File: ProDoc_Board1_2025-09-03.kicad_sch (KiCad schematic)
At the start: 47 parts, among them CN10 BATT, CN11 CHGIN, CN2 B04B-XNISK-A-1(LF)(SN), CN3 B04B-XNISK-A-1(LF)(SN), CN4 B04B-XNISK-A-1(LF)(SN), CN7 XH2.54-5PIN, CN8 A2502-WV02, CN9 A2502-WV02, J1 Conn_01x05_Pin, J2 Conn_01x02_Pin, U1 MAX77961EFV06+, U3 Ra-02, U4 XL 4005

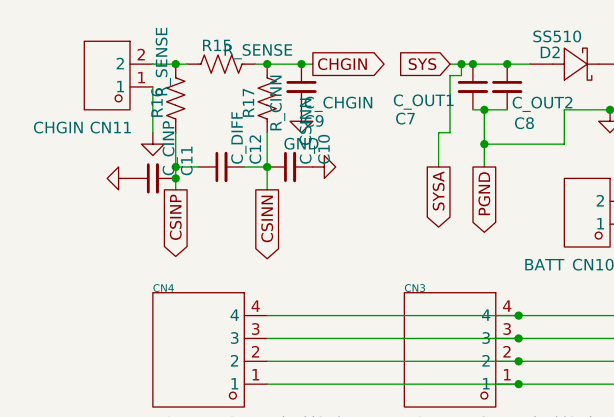
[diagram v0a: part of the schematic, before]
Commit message: layout started
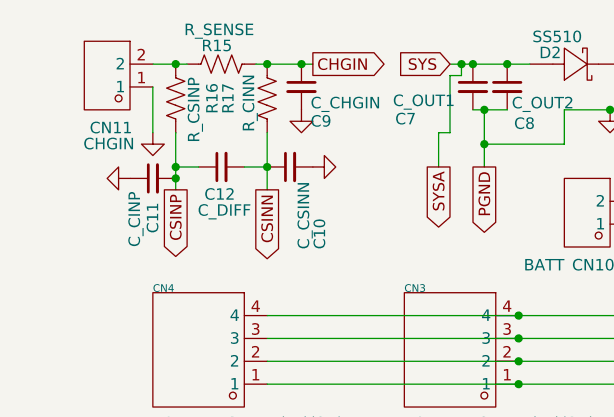
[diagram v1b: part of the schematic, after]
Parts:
- C10, C11, C12: footprint Capacitor_SMD:C_1210_3225Metric -> Capacitor_SMD:C_0402_1005Metric
- C7, C8: footprint Capacitor_SMD:C_1210_3225Metric_Pad1.33x2.70mm_HandSolder -> Capacitor_SMD:C_1210_3225Metric
- CN10, CN11: footprint Connector_JST:JST_SH_BM02B-SRSS-TB_1x02-1MP_P1.00mm_Vertical -> Connector_JST:JST_VH_B2P-VH_1x02_P3.96mm_Vertical
- R16: value R_SENSE -> R_CSINP; footprint Resistor_SMD:R_1206_3216Metric -> Resistor_SMD:R_0402_1005Metric
- R17: footprint Resistor_SMD:R_1206_3216Metric -> Resistor_SMD:R_0402_1005Metric
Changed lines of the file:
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@@
 			)
 		)
-		(property "Footprint" "Capacitor_SMD:C_1210_3225Metric_Pad1.33x2.70mm_HandSolder"
+		(property "Footprint" "Capacitor_SMD:C_1210_3225Metric"
 			(at 60.96 26.67 0)
 			(effects
@@
 			)
 		)
-		(property "Footprint" "Connector_JST:JST_SH_BM02B-SRSS-TB_1x02-1MP_P1.00mm_Vertical"
+		(property "Footprint" "Connector_JST:JST_VH_B2P-VH_1x02_P3.96mm_Vertical"
 			(at 69.85 40.64 0)
 			(effects
@@
 		(dnp no)
 		(property "Reference" "R17"
-			(at 32.258 28.448 90)
+			(at 29.972 27.94 90)
 			(effects
 				(font
@@
 		)
 		(property "Value" "R_CINN"
-			(at 35.306 28.448 90)
+			(at 32.258 28.448 90)
 			(effects
 				(font
@@
 			)
 		)
-		(property "Footprint" "Resistor_SMD:R_1206_3216Metric"
+		(property "Footprint" "Resistor_SMD:R_0402_1005Metric"
 			(at 33.274 27.686 90)
 			(effects
@@
 		(dnp no)
 		(property "Reference" "C9"
-			(at 38.354 30.4862 0)
+			(at 39.116 30.4862 0)
 			(effects
 				(font
@@
 		)
 		(property "Value" "C_CHGIN"
-			(at 38.354 28.4542 0)
+			(at 39.116 28.4542 0)
 			(effects
 				(font
@@
 		(dnp no)
 		(property "Reference" "C10"
-			(at 40.6462 35.306 0)
+			(at 40.1382 44.704 0)
 			(effects
 				(font
@@
 		)
 		(property "Value" "C_CSINN"
-			(at 38.6142 35.306 0)
+			(at 38.3602 44.704 0)
 			(effects
 				(font
@@
 			)
 		)
-		(property "Footprint" "Capacitor_SMD:C_1210_3225Metric"
+		(property "Footprint" "Capacitor_SMD:C_0402_1005Metric"
 			(at 36.83 35.56 0)
 			(effects
@@
 		(dnp no)
 		(property "Reference" "C11"
-			(at 25.4062 36.576 0)
+			(at 21.5962 42.926 0)
 			(effects
 				(font
@@
 		)
 		(property "Value" "C_CINP"
-			(at 23.3742 36.576 0)
+			(at 19.5642 44.45 0)
 			(effects
 				(font
@@
 			)
 		)
-		(property "Footprint" "Capacitor_SMD:C_1210_3225Metric"
+		(property "Footprint" "Capacitor_SMD:C_0402_1005Metric"
 			(at 21.59 36.83 0)
 			(effects
@@
 		(dnp no)
 		(property "Reference" "C12"
-			(at 33.0262 35.306 0)
+			(at 30.7402 38.608 90)
 			(effects
 				(font
@@
 		)
 		(property "Value" "C_DIFF"
-			(at 30.9942 35.306 0)
+			(at 32.5182 40.386 90)
 			(effects
 				(font
@@
 			)
 		)
-		(property "Footprint" "Capacitor_SMD:C_1210_3225Metric"
+		(property "Footprint" "Capacitor_SMD:C_0402_1005Metric"
 			(at 29.21 35.56 0)
 			(effects
@@
 		)
 		(property "Value" "R_SENSE"
-			(at 33.274 22.606 90)
+			(at 28.956 20.32 90)
 			(effects
 				(font
@@
 					(size 1.27 1.27)
 				)
+				(hide yes)
 			)
 		)
@@
 		)
 		(property "Value" "CHGIN"
-			(at 13.97 30.48 0)
+			(at 19.558 32.258 0)
 			(effects
 				(font
@@
 			)
 		)
-		(property "Footprint" "Connector_JST:JST_SH_BM02B-SRSS-TB_1x02-1MP_P1.00mm_Vertical"
+		(property "Footprint" "Connector_JST:JST_VH_B2P-VH_1x02_P3.96mm_Vertical"
 			(at 16.51 25.4 0)
 			(effects
@@
 		(dnp no)
 		(property "Reference" "R16"
-			(at 22.098 28.448 90)
+			(at 28.194 27.94 90)
 			(effects
 				(font
@@
 			)
 		)
-		(property "Value" "R_SENSE"
-			(at 22.606 23.876 90)
+		(property "Value" "R_CSINP"
+			(at 26.162 29.21 90)
 			(effects
 				(font
@@
 			)
 		)
-		(property "Footprint" "Resistor_SMD:R_1206_3216Metric"
+		(property "Footprint" "Resistor_SMD:R_0402_1005Metric"
 			(at 23.114 27.686 90)
 			(effects
@@
 			)
 		)
-		(property "Footprint" "Capacitor_SMD:C_1210_3225Metric_Pad1.33x2.70mm_HandSolder"
+		(property "Footprint" "Capacitor_SMD:C_1210_3225Metric"
 			(at 57.15 26.67 0)
 			(effects
